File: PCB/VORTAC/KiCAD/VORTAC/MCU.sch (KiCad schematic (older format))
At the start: 42 parts, among them IC1 TMC2209-LA, U2 STM32F103C8Tx, U5 ADXL345BCCZ-RL, U6 SN65HVD232DR

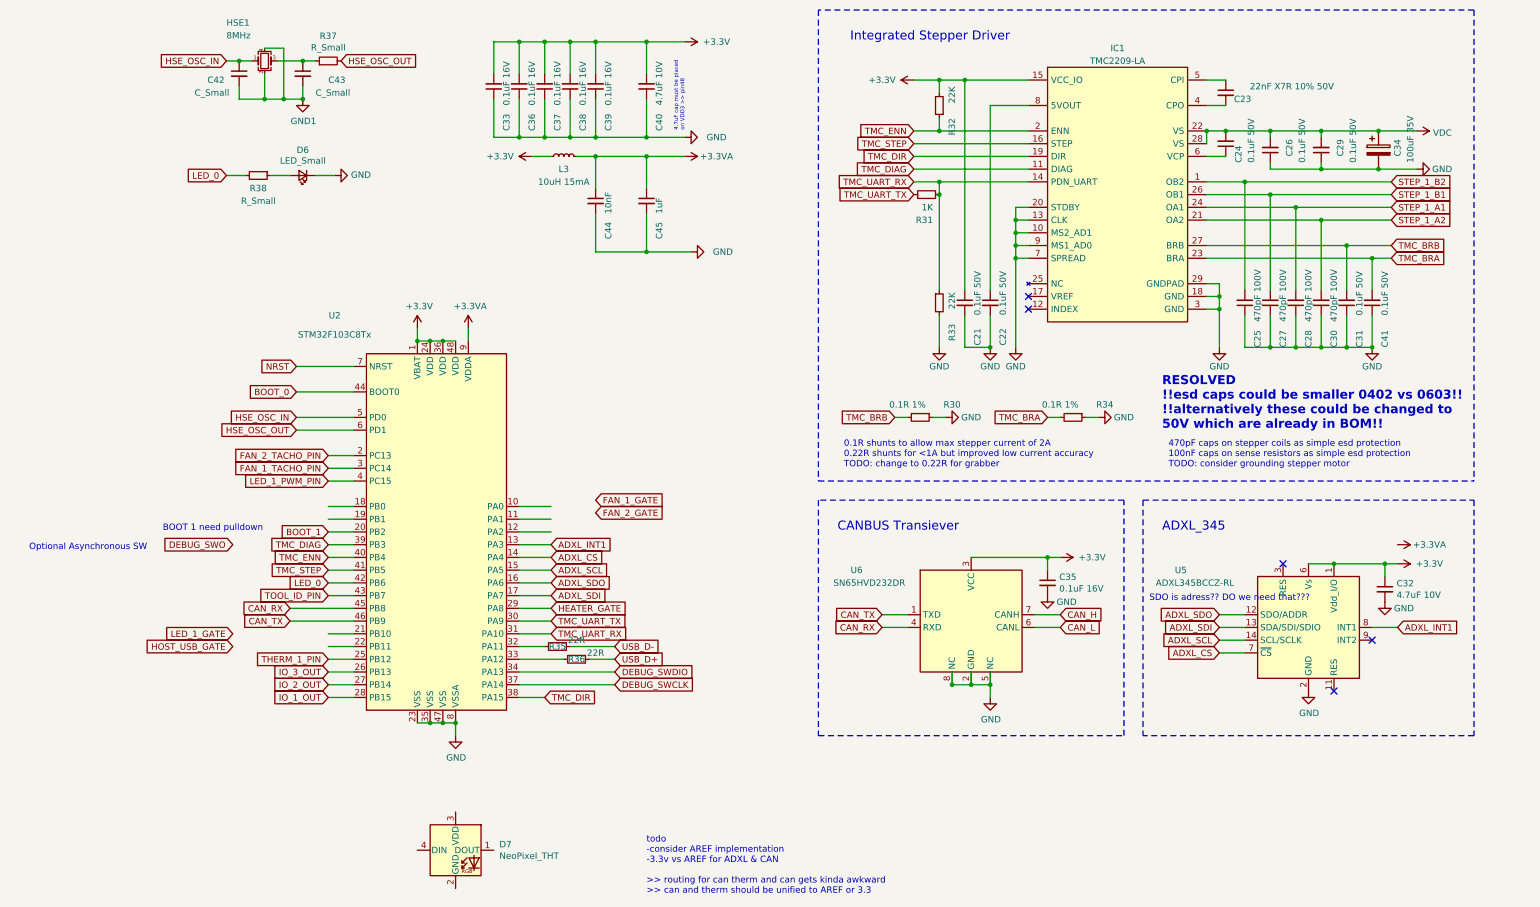
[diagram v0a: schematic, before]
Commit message: pushy
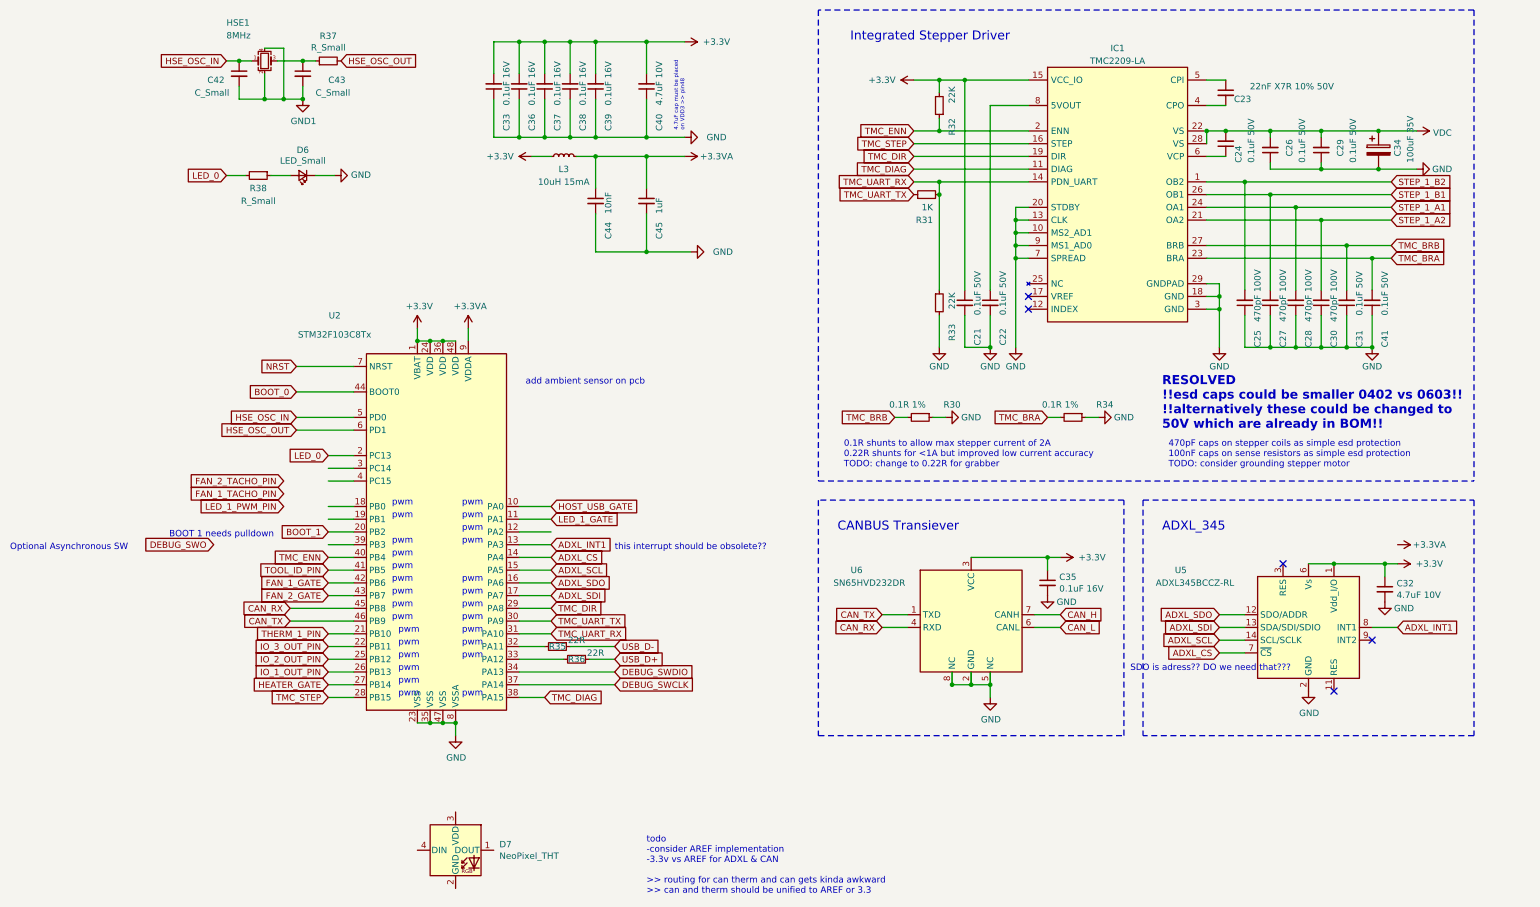
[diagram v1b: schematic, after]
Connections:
- net labels added: IO_1_OUT_PIN, IO_2_OUT_PIN, IO_3_OUT_PIN
- net labels removed: IO_1_OUT, IO_2_OUT, IO_3_OUT
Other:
- note added: "BOOT 1 needs pulldown"
- note added: "add ambient sensor on pcb\n"
- note added: "pwm"
- note added: "this interrupt should be obsolete??"
- note removed: "BOOT 1 need pulldown"
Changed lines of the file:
@@
 	2050 5550 2250 5550
-Wire Wire Line
-	2050 5650 2250 5650
 Wire Wire Line
 	3550 4750 3800 4750
@@
 Text GLabel 4300 5950 2    50   Input ~ 0
 DEBUG_SWCLK
-Text GLabel 1300 4850 0    50   Input ~ 0
+Text GLabel 1150 4850 0    50   Input ~ 0
 DEBUG_SWO
 Wire Wire Line
 	2050 4850 2250 4850
-Text Notes -300 4900 0    50   ~ 0
+Text Notes -450 4900 0    50   ~ 0
 Optional Asynchronous SW
 Wire Wire Line
@@
 Wire Wire Line
 	2050 4650 2250 4650
-Text GLabel 3750 6050 2    50   Input ~ 0
+Text GLabel 3800 5350 2    50   Input ~ 0
 TMC_DIR
-Text GLabel 2050 5050 0    50   Input ~ 0
+Text GLabel 2050 6050 0    50   Input ~ 0
 TMC_STEP
 Text GLabel 2050 4950 0    50   Input ~ 0
 TMC_ENN
-Text GLabel 2050 4850 0    50   Input ~ 0
+Text GLabel 3750 6050 2    50   Input ~ 0
 TMC_DIAG
-Text GLabel 2050 4250 0    50   Input ~ 0
+Text GLabel 1700 4450 0    50   Input ~ 0
 FAN_1_TACHO_PIN
-Text GLabel 2050 4150 0    50   Input ~ 0
+Text GLabel 1700 4350 0    50   Input ~ 0
 FAN_2_TACHO_PIN
-Text GLabel 4150 4600 2    50   Input ~ 0
-FAN_2_GATE
-Text GLabel 3800 5350 2    50   Input ~ 0
+Text GLabel 2050 5950 0    50   Input ~ 0
 HEATER_GATE
-Text GLabel 1300 5550 0    50   Input ~ 0
+Text GLabel 3800 4650 2    50   Input ~ 0
 LED_1_GATE
-Text GLabel 1300 5650 0    50   Input ~ 0
+Text GLabel 3800 4550 2    50   Input ~ 0
 HOST_USB_GATE
-Text GLabel 2050 5150 0    50   Input ~ 0
-LED_0
 Text GLabel 3800 4950 2    50   Input ~ 0
 ADXL_CS
@@
 Text GLabel 3800 4850 2    50   Input ~ 0
 ADXL_INT1
-Text GLabel 2050 5250 0    50   Input ~ 0
-TOOL_ID_PIN
-Text GLabel 2050 5750 0    50   Input ~ 0
-THERM_1_PIN
-Text GLabel 2050 5850 0    50   Input ~ 0
-IO_3_OUT
-Text GLabel 2050 5950 0    50   Input ~ 0
-IO_2_OUT
-Text GLabel 2050 6050 0    50   Input ~ 0
-IO_1_OUT
 $Comp
 L Device:LED_Small D6
@@
 Wire Wire Line
 	3550 5850 4300 5850
-Text GLabel 4150 4500 2    50   Input ~ 0
-FAN_1_GATE
-Text GLabel 2050 4350 0    50   Input ~ 0
+Text GLabel 1700 4550 0    50   Input ~ 0
 LED_1_PWM_PIN
 Wire Wire Line
@@
 Wire Wire Line
 	2050 4750 2250 4750
-Text Notes 8500 5300 0    50   ~ 0
-SDO is adress?? DO we need that???
-Wire Wire Line
-	2050 5750 2250 5750
-Wire Wire Line
-	2050 5850 2250 5850
-Wire Wire Line
-	2050 5950 2250 5950
-Wire Wire Line
-	2050 6050 2250 6050
 Wire Wire Line
 	2050 4950 2250 4950
@@
 	1    0    0    -1
 $EndComp
-Text Notes 750  4750 0    50   ~ 0
-BOOT 1 need pulldown
+Text Notes 800  4800 0    50   ~ 0
+BOOT 1 needs pulldown
+Text GLabel 2050 5150 0    50   Input ~ 0
+FAN_1_GATE
+Text GLabel 2050 4150 0    50   Input ~ 0
+LED_0
+Text GLabel 2050 5250 0    50   Input ~ 0
+FAN_2_GATE
+Text GLabel 2050 5050 0    50   Input ~ 0
+TOOL_ID_PIN
+Wire Wire Line
+	2050 6050 2250 6050
+Wire Wire Line
+	2050 5950 2250 5950
+Wire Wire Line
+	2050 5850 2250 5850
+Wire Wire Line
+	2050 5750 2250 5750
+Text GLabel 2050 5850 0    50   Input ~ 0
+IO_1_OUT_PIN
+Text GLabel 2050 5750 0    50   Input ~ 0
+IO_2_OUT_PIN
+Text GLabel 2050 5650 0    50   Input ~ 0
+IO_3_OUT_PIN
+Text GLabel 2050 5550 0    50   Input ~ 0
+THERM_1_PIN
+Wire Wire Line
+	2050 5650 2250 5650
+Text Notes 8350 5850 0    50   ~ 0
+SDO is adress?? DO we need that???
+Text Notes 3600 3600 0    50   ~ 0
+add ambient sensor on pcb\n
+Text Notes 2550 4550 0    50   ~ 0
+pwm
+Text Notes 2550 4650 0    50   ~ 0
+pwm
+Text Notes 2600 5550 0    50   ~ 0
+pwm
+Text Notes 2600 5650 0    50   ~ 0
+pwm
+Text Notes 2600 5750 0    50   ~ 0
+pwm
+Text Notes 2600 5850 0    50   ~ 0
+pwm
+Text Notes 2600 5950 0    50   ~ 0
+pwm
+Text Notes 2600 6050 0    50   ~ 0
+pwm
+Text Notes 3100 5350 0    50   ~ 0
+pwm
+Text Notes 3100 5450 0    50   ~ 0
+pwm
+Text Notes 3100 5550 0    50   ~ 0
+pwm
+Text Notes 3100 5650 0    50   ~ 0
+pwm
+Text Notes 3100 5750 0    50   ~ 0
+pwm
+Text Notes 3100 6050 0    50   ~ 0
+pwm
+Text Notes 2550 4850 0    50   ~ 0
+pwm
+Text Notes 2550 4950 0    50   ~ 0
+pwm
+Text Notes 2550 5050 0    50   ~ 0
+pwm
+Text Notes 2550 5150 0    50   ~ 0
+pwm
+Text Notes 2550 5250 0    50   ~ 0
+pwm
+Text Notes 2550 5350 0    50   ~ 0
+pwm
+Text Notes 2550 5450 0    50   ~ 0
+pwm
+Text Notes 3100 4550 0    50   ~ 0
+pwm
+Text Notes 3100 4650 0    50   ~ 0
+pwm
+Text Notes 3100 4750 0    50   ~ 0
+pwm
+Text Notes 3100 4850 0    50   ~ 0
+pwm
+Text Notes 3100 5150 0    50   ~ 0
+pwm
+Text Notes 3100 5250 0    50   ~ 0
+pwm
+Text Notes 4300 4900 0    50   ~ 0
+this interrupt should be obsolete??
 $EndSCHEMATC
